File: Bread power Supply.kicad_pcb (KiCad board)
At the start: 2 copper layers, 32.5 x 53.3 mm, 18 parts, among them J1 01x02_Pin, J2 01x02_Pin, J3 Conn_01x03_Pin, J4 Conn_01x03_Pin, J5 Screw_Terminal_01x02, J6 Barrel_Jack_Switch, J7 Screw_Terminal_01x02, U1 LM7805_TO220, U2 LM317_TO-220

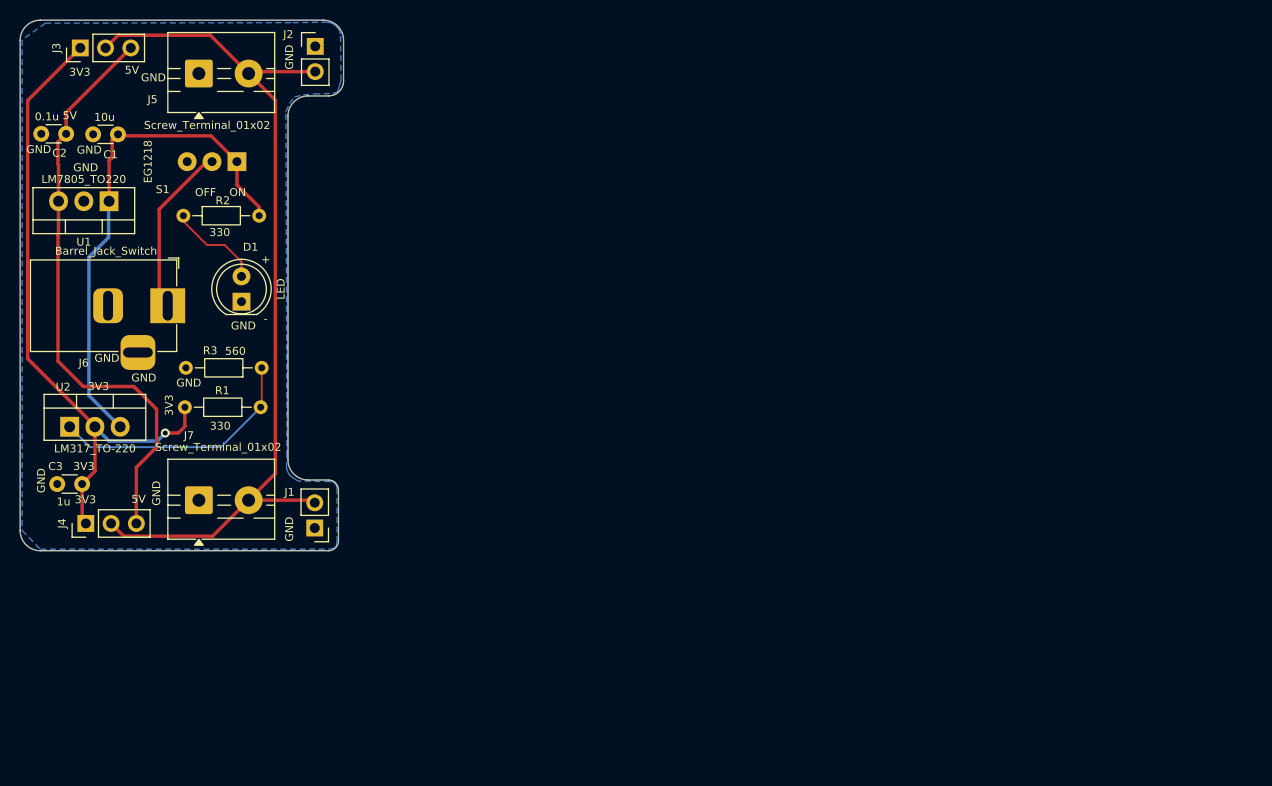
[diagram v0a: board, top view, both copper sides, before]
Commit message: update
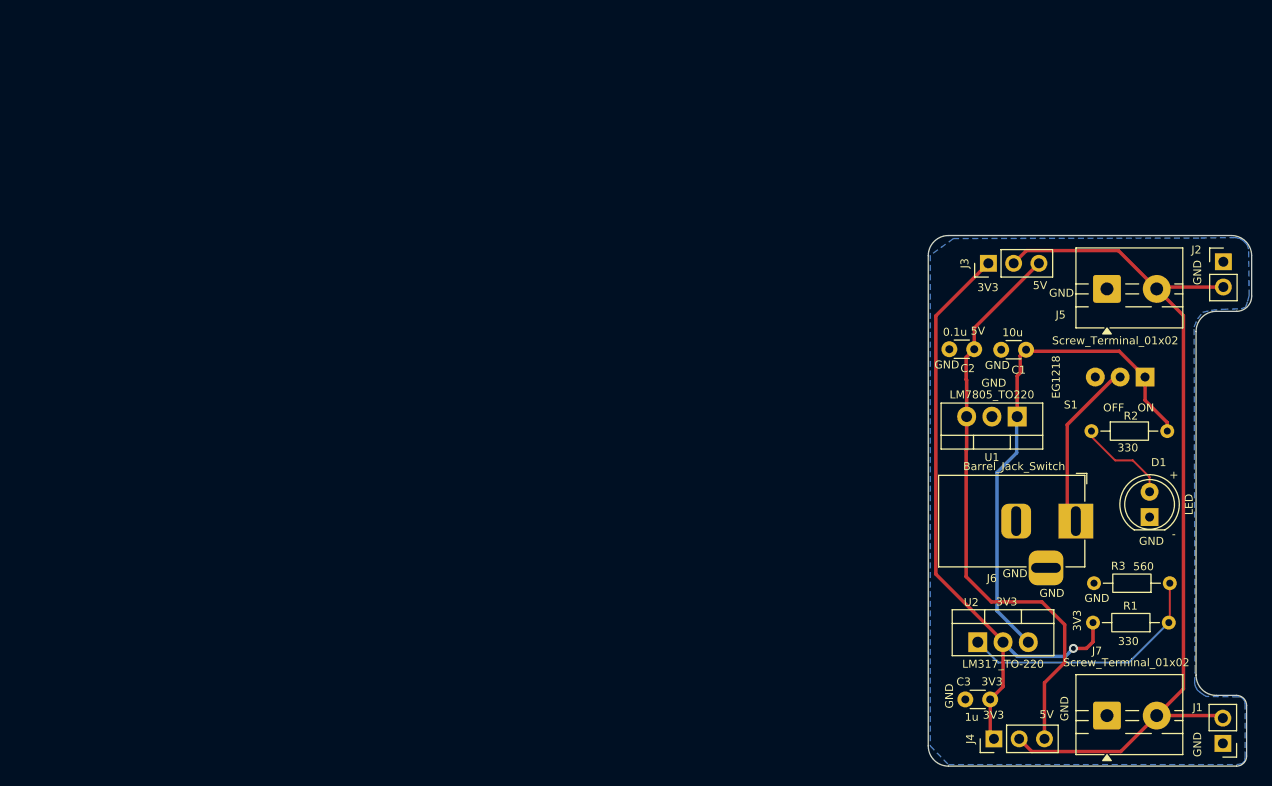
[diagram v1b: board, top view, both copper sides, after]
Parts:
- moved J1 93.8 mm to (163.1, 150.4)
- moved R2 93.8 mm to (149.9, 119.0)
- moved R3 93.8 mm to (157.7, 134.3)
- moved U1 93.8 mm to (142.4, 117.6)
- moved C1 93.8 mm to (143.3, 110.9)
- moved C2 93.8 mm to (138.1, 110.8)
- moved C3 93.8 mm to (137.2, 146.0)
- moved D1 93.8 mm to (155.7, 127.7)
- moved J2 93.8 mm to (163.1, 102.0)
- moved J3 93.8 mm to (139.5, 102.2)
- moved J4 93.8 mm to (140.1, 150.0)
- moved J5 93.8 mm to (151.4, 104.7)
- moved J6 93.8 mm to (148.3, 128.1)
- moved J7 93.8 mm to (151.4, 147.6)
- moved REF** 93.8 mm to (137.4, 126.8)
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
